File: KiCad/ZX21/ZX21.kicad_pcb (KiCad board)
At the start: 2 copper layers, 142 x 100 mm, 131 parts, among them IC1 ULA 2C210E, IC101 555, IC102 74HCT00, IC2 AT28C256, IC3 Z80A, IC301 3V3 PSU, IC302 ESP32-WROOM, IC303 AZ1117-3.3, IC4 62256, IC501 YM2149, IC502 GAL16V8, IC503 YMZ284, IC801 AS6C4008Extra, J1 Jack-DC, J101 Conn_01x03, J203 Conn_01x03, J204 Conn_01x03, J301 Conn_01x04, J302 Conn_01x03, J401 DB9_Male, J501 Conn_01x06, J502 Conn_01x08, J503 Conn_01x08, J504 Conn_01x08, J601 Conn_02x08_Odd_Even, J701 Conn_02x23_Row_Letter_First, J702 Conn_01x09, J703 Conn_01x09, X1 3.5MHz

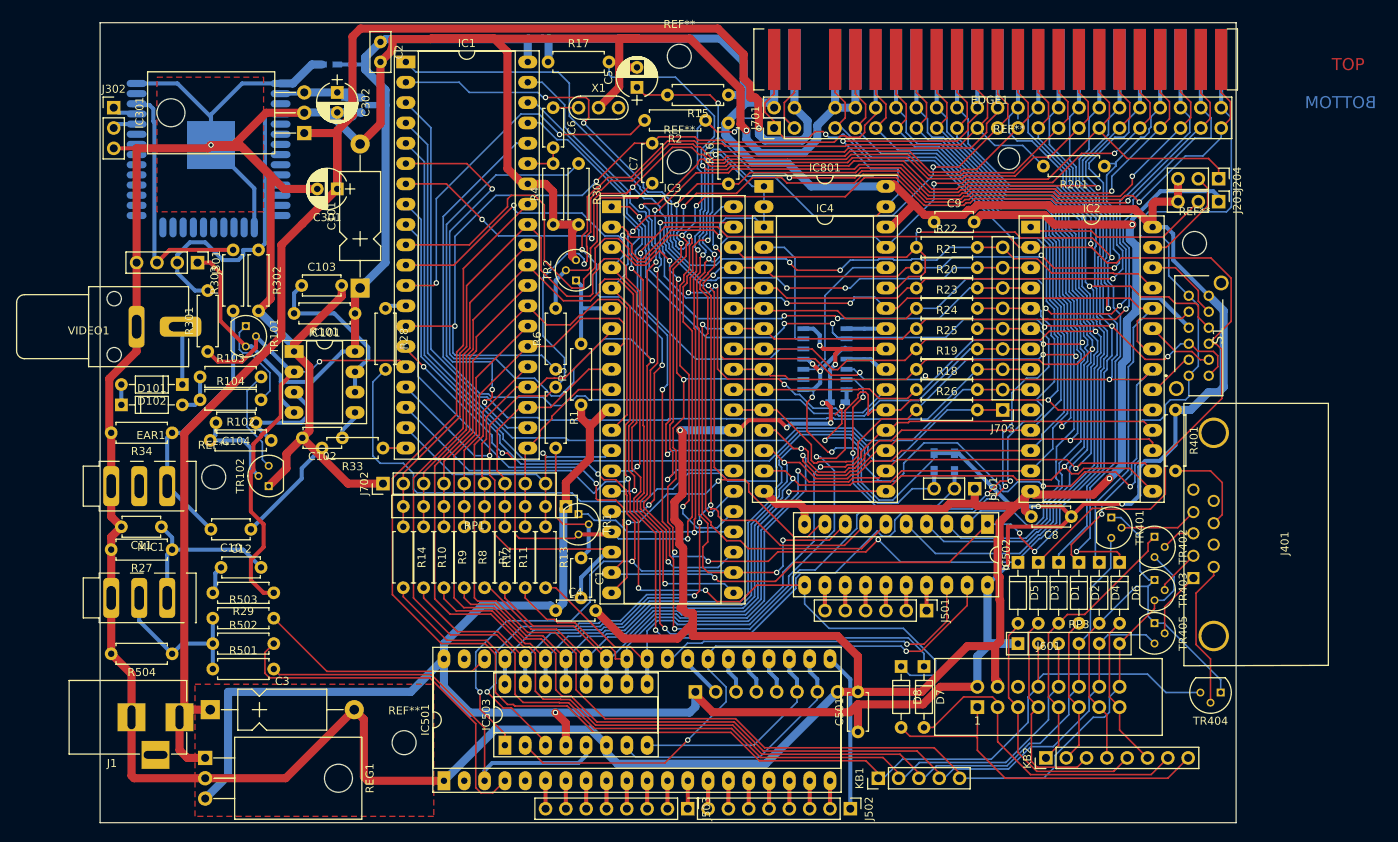
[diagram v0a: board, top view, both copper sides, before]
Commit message: Fixing DRC Issues
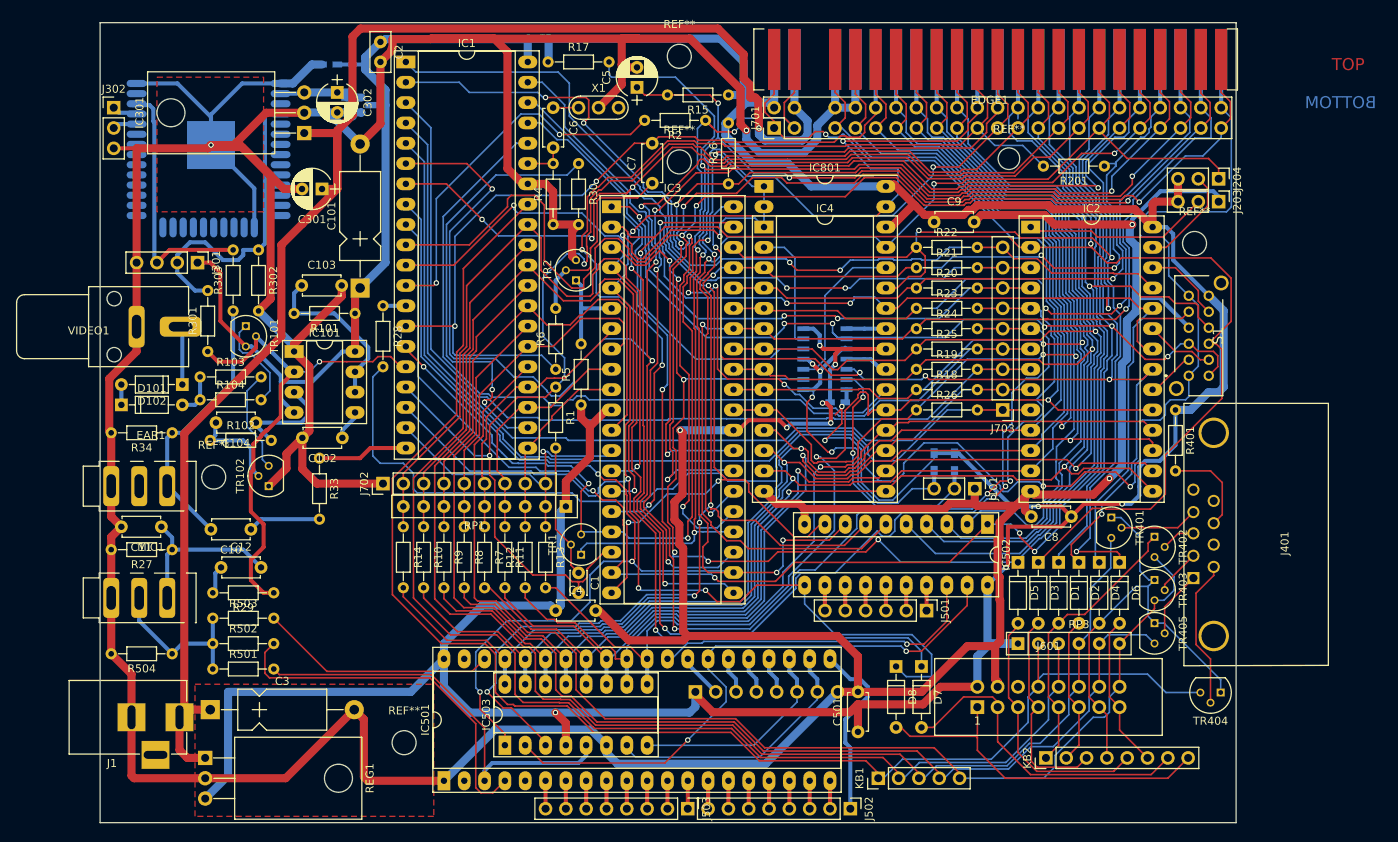
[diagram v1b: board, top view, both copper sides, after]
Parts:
- C1: footprint Capacitors_THT:C_Disc_D4.7mm_W2.5mm_P5.00mm -> Capacitors_THT:C_Disc_D3.0mm_W2.0mm_P2.50mm
- C10, C102, C103, C104, C11, C12, C4, C501, C6, C7, C8, C9: footprint Capacitors_THT:C_Disc_D4.7mm_W2.5mm_P5.00mm -> Capacitors_ThroughHole:C_Disc_D4.7mm_W2.5mm_P5.00mm
- C3: footprint Capacitors_THT:CP_Axial_L11.0mm_D5.0mm_P18.00mm_Horizontal -> Capacitors_ThroughHole:CP_Axial_L11.0mm_D5.0mm_P18.00mm_Horizontal
- C301, C302, C5: footprint Capacitors_THT:CP_Radial_D5.0mm_P2.50mm -> Capacitors_ThroughHole:CP_Radial_D5.0mm_P2.50mm
- D1, D101, D102, D2, D3, D4, D5, D6, D7, D8: footprint Diodes_THT:D_DO-35_SOD27_P7.62mm_Horizontal -> zxbus:D_DO-35_SOD27_P7.62mm_Horizontal
- R1, R10, R101, R102, R103, R104, R11, R12, R13, R14, R15, R16, R17, R18, R19, R2, R20, R201, R21, R22, R23, R24, R25, R26, R27, R28, R29, R30, R301, R302, R303, R33, R34, R4, R401, R5, R501, R502, R503, R504, R6, R7, R8, R9: footprint Resistors_ThroughHole:R_Axial_DIN0207_L6.3mm_D2.5mm_P7.62mm_Horizontal -> Resistors_ThroughHole:R_Axial_DIN0204_L3.6mm_D1.6mm_P7.62mm_Horizontal
- moved R33 8.04 mm to (58.4, 91.4), turned to 270 degrees
- moved TR1 5.09 mm to (91.1, 103.5), turned to 90 degrees
- moved C301 1.91 mm to (58.7, 57.8)
- moved C1 1.89 mm to (90.8, 105.8)
- moved D8 0.63 mm to (130.5, 117.5)
- moved R28 0.45 mm to (66.4, 72.4)
- moved D7 0.32 mm to (133.7, 117.5)
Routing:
- net Net-(IC1-Pad20): track 2.86 -> 11.3 mm
- net Net-(C10-Pad1): track 13.8 -> 9.10 mm
- net Net-(IC501-Pad21): track 19.8 -> 22.9 mm
- net GND: track 827.6 -> 824.8 mm
- net +9V: track 195.7 -> 197.6 mm
- net HALT: track 163.0 -> 161.2 mm
- net MREQ: track 190.0 -> 188.9 mm
- net A15: track 203.6 -> 204.6 mm
- net Net-(C1-Pad1): track 17.7 -> 16.8 mm

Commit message: Fixing DRC Issues
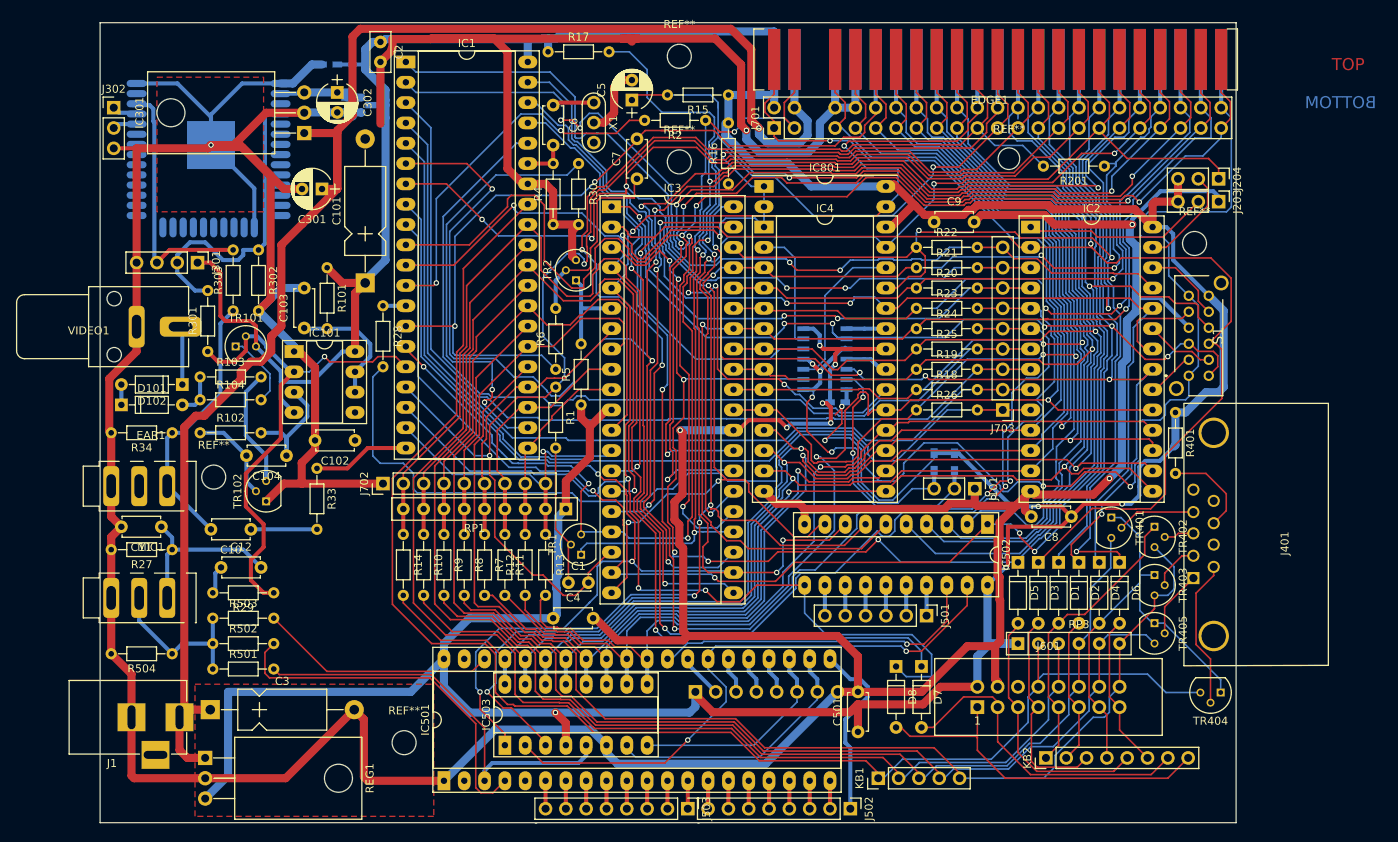
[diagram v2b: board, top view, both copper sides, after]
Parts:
- J502, J503, J504: footprint Pin_Headers:Pin_Header_Straight_1x08_Pitch2.54mm -> zxbus:Pin_Header_Straight_1x08_Pitch2.54mm
- moved R101 6.70 mm to (59.4, 67.6), turned to 270 degrees
- moved C104 5.62 mm to (54.3, 91.1)
- moved C103 5.33 mm to (56.5, 75.2), turned to 90 degrees
- moved TR101 2.84 mm to (47.9, 77.5), turned to 0 degrees
- moved X1 2.01 mm to (92.7, 47.0), turned to 270 degrees
- moved C7 1.98 mm to (98.1, 56.5)
- moved TR102 1.93 mm to (51.8, 96.8)
- moved C1 1.77 mm to (89.5, 107.0), turned to 0 degrees
- moved C5 1.71 mm to (97.5, 46.7)
- moved C102 1.62 mm to (62.9, 89.2)
- moved R102 1.59 mm to (43.5, 88.3)
- moved R33 1.31 mm to (58.1, 92.7)
- moved R17 1.27 mm to (87.0, 40.6)
- moved TR402 1.25 mm to (162.8, 100.0)
- moved C4 1.00 mm to (87.6, 111.4)
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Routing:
- net GND: track 824.8 -> 812.2 mm
- net +5V: track 553.5 -> 561.0 mm
- net Net-(C103-Pad1): track 21.2 -> 15.9 mm
- net Net-(R103-Pad2): track 12.9 -> 17.3 mm
- net Net-(C102-Pad1): track 3.83 -> 0.00 mm
- net Net-(R104-Pad2): track 12.1 -> 9.40 mm
- net +9V: track 197.6 -> 199.8 mm
- net KBD4: track 151.7 -> 153.9 mm
- net IORQ: track 192.9 -> 195.1 mm
- net Net-(C6-Pad1): track 3.18 -> 5.21 mm
- net D7': track 186.6 -> 188.6 mm
- net Net-(C104-Pad1): track 13.5 -> 15.5 mm
- net A8': track 113.7 -> 115.6 mm
- net A5': track 160.3 -> 162.1 mm
- net A6': track 83.3 -> 85.1 mm
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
